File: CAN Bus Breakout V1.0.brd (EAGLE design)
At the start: 50 x 50 mm, 33 parts, among them U1 HEX_CONVERTER

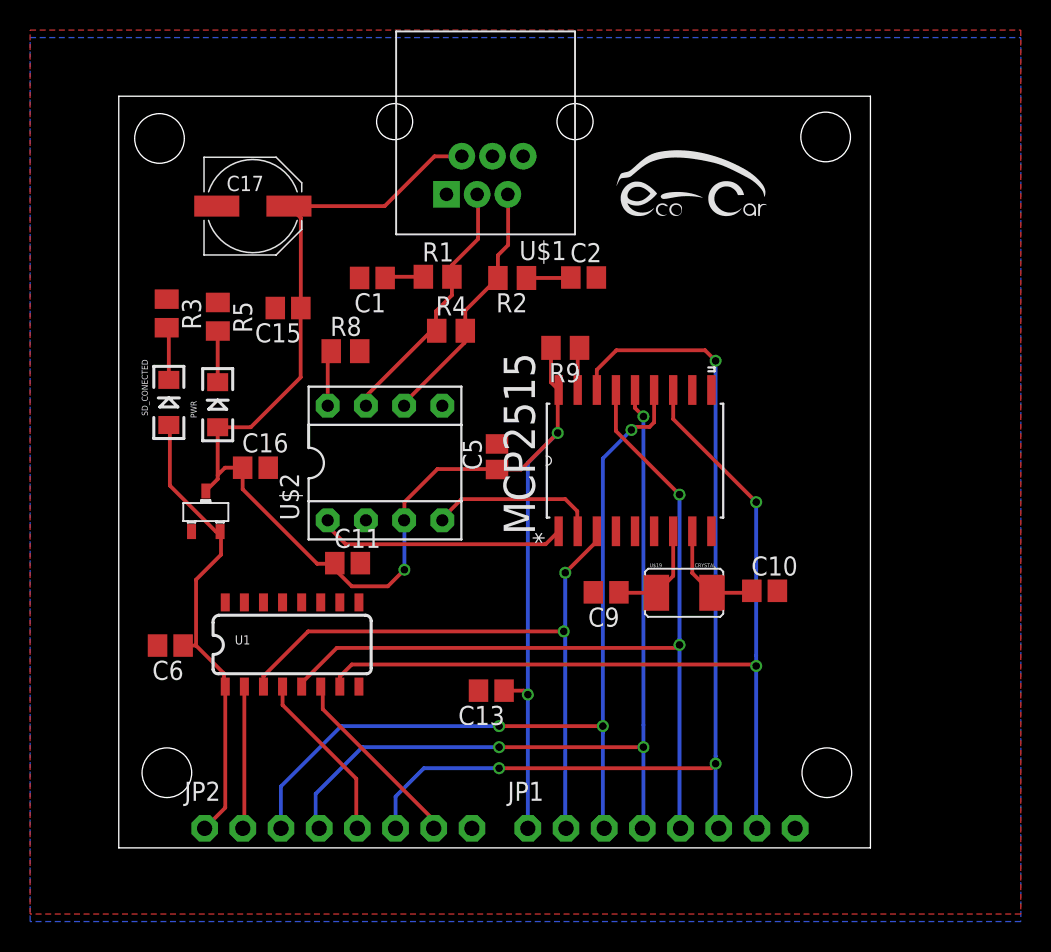
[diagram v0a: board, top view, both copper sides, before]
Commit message: Complete
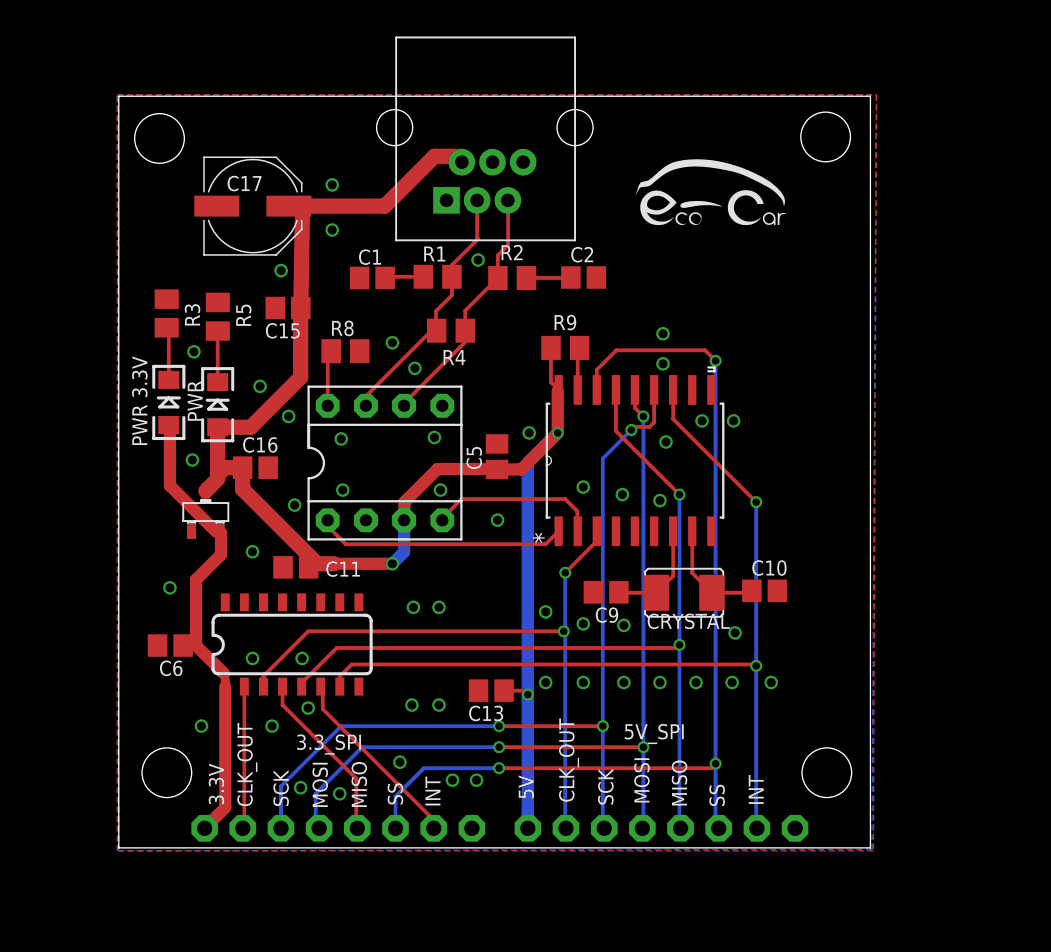
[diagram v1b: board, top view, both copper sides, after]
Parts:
- moved C11 3.45 mm to (11.8, 18.7), turned to 180 degrees
- moved U$3 1.43 mm to (39.8, 43.2)
- moved U$1 0.40 mm to (25.9, 43.1)
- renumbered JP1 to 5V_SPI, JP2 to 3.3_SPI
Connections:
- removed net N$10: U1.10
- removed net N$13: U1.9
- net GND: now also U1.11, U1.14, U1.9
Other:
- board text added: "3.3V"
- board text added: "5V"
- board text added: "CLK_OUT"
- board text added: "INT"
- board text added: "MISO"
- board text added: "MOSI"
- board text added: "PWR 3.3V"
- board text added: "SCK"
- board text added: "SS"
